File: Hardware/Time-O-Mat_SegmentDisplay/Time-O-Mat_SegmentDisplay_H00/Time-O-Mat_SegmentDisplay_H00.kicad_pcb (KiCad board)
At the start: 2 copper layers, 55.1 x 132.3 mm, 45 parts, among them J1 Conn_02x04_Odd_Even

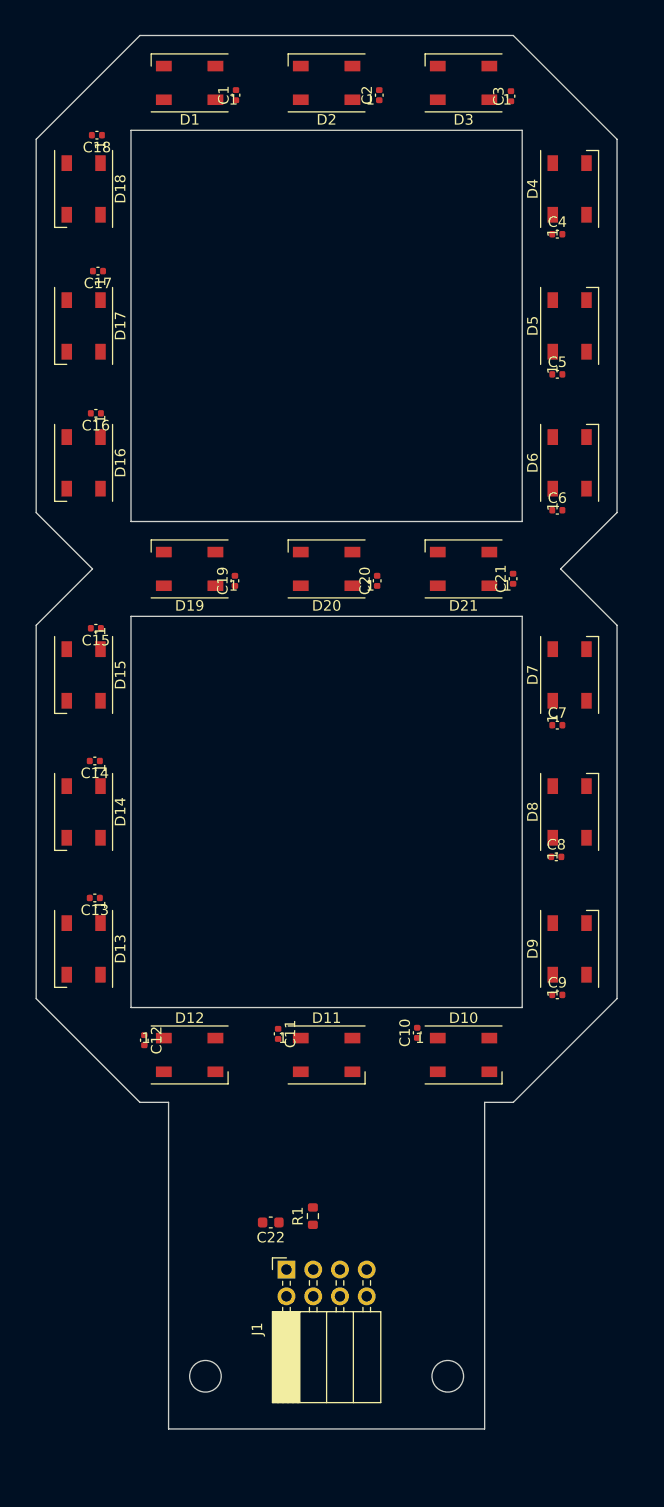
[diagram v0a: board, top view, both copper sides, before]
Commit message: Updated segment pcb
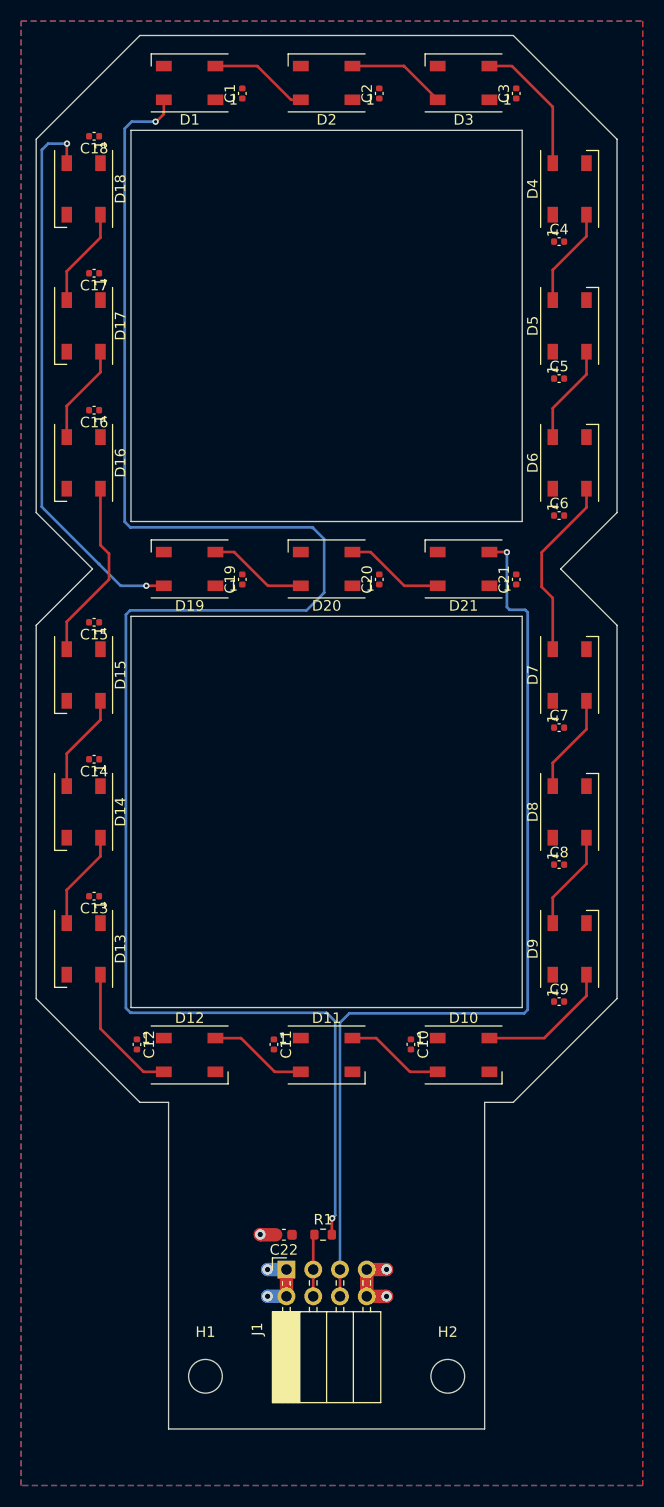
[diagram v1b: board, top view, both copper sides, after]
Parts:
- added H1: MountingHole, MountingHole:MountingHole_3.2mm_M3, F.Cu at (-11.5, 76.6)
- added H2: MountingHole, MountingHole:MountingHole_3.2mm_M3, F.Cu at (11.5, 76.6)
- moved R1 2.01 mm to (-0.33, 63.2), turned to 0 degrees
- moved C22 1.71 mm to (-4.05, 63.2)
- moved C10 1.25 mm to (8.00, 45.1), turned to -90 degrees
- moved C11 1.08 mm to (-5.00, 45.1)
- moved C12 0.81 mm to (-18.0, 45.1)
- moved C8 0.78 mm to (22.1, 28.1)
- moved C4 0.72 mm to (22.1, -31.1)
- moved C19 0.71 mm to (-8.00, 1.00)
- moved C9 0.66 mm to (22.1, 41.1)
- moved C1 0.62 mm to (-8.00, -45.1)
- moved C15 0.59 mm to (-22.1, 5.07)
- moved C3 0.56 mm to (18.0, -45.1)
- moved C6 0.53 mm to (22.1, -5.07)
- moved C5 0.44 mm to (22.1, -18.1)
- moved C17 0.42 mm to (-22.1, -28.1)
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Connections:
- net Net-(C22-Pad1) renamed +5V
- net Net-(C22-Pad2) renamed GND
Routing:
- net Net-(D1-Pad4): track 0.00 -> 165.5 mm, vias 0 -> 2
- net Net-(D21-Pad2): track 0.00 -> 91.1 mm, vias 0 -> 1
- net Net-(D18-Pad2): track 0.00 -> 53.1 mm, vias 0 -> 2
- net Net-(D6-Pad2): track 0.00 -> 17.4 mm
- net Net-(D15-Pad2): track 0.00 -> 17.2 mm
- net Net-(D3-Pad2): track 0.00 -> 13.0 mm
- net Net-(D10-Pad4): track 0.00 -> 12.9 mm
- net Net-(D12-Pad2): track 0.00 -> 12.8 mm
- net Net-(D2-Pad2): track 0.00 -> 9.43 mm
- net Net-(D11-Pad2): track 0.00 -> 9.43 mm
- net Net-(D10-Pad2): track 0.00 -> 9.43 mm
- net Net-(D1-Pad2): track 0.00 -> 9.43 mm
- net Net-(D7-Pad2): track 0.00 -> 9.43 mm
- net Net-(D5-Pad2): track 0.00 -> 9.43 mm
- net Net-(D20-Pad2): track 0.00 -> 9.43 mm
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- added copper zone on F.Cu, net +5V
- added copper zone on B.Cu, net GND
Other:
- outline, holes or cut-outs redrawn
